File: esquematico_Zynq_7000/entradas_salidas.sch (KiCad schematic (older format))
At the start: 41 parts, among them U5 XC7Z010

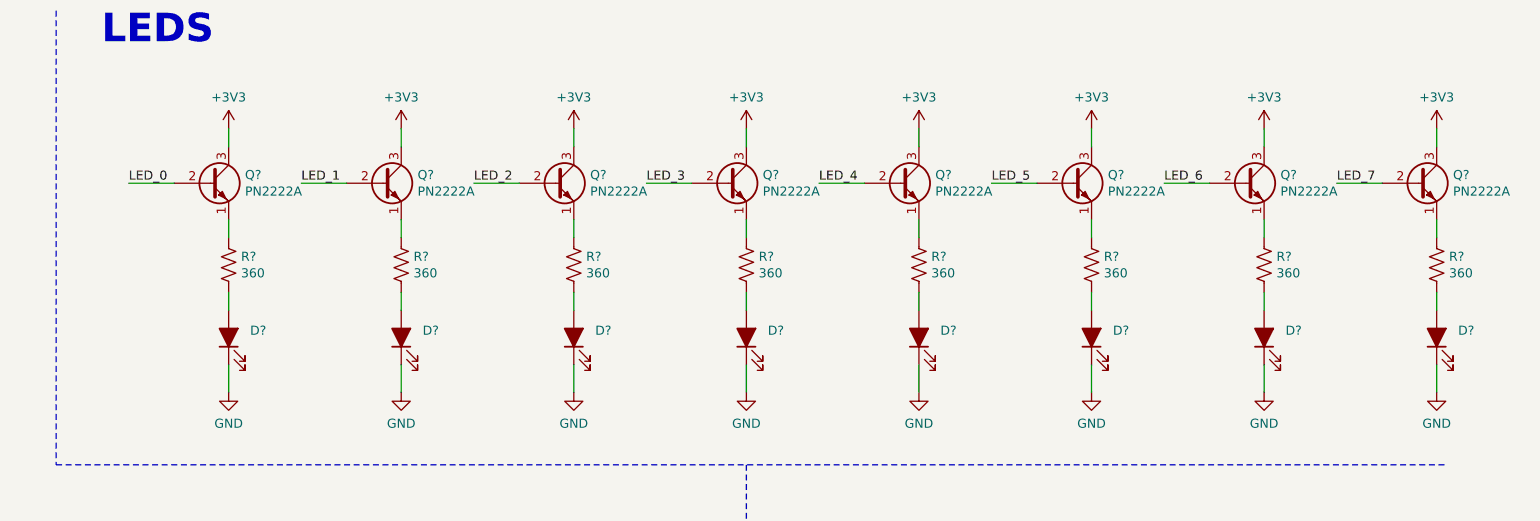
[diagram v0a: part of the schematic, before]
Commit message: upd
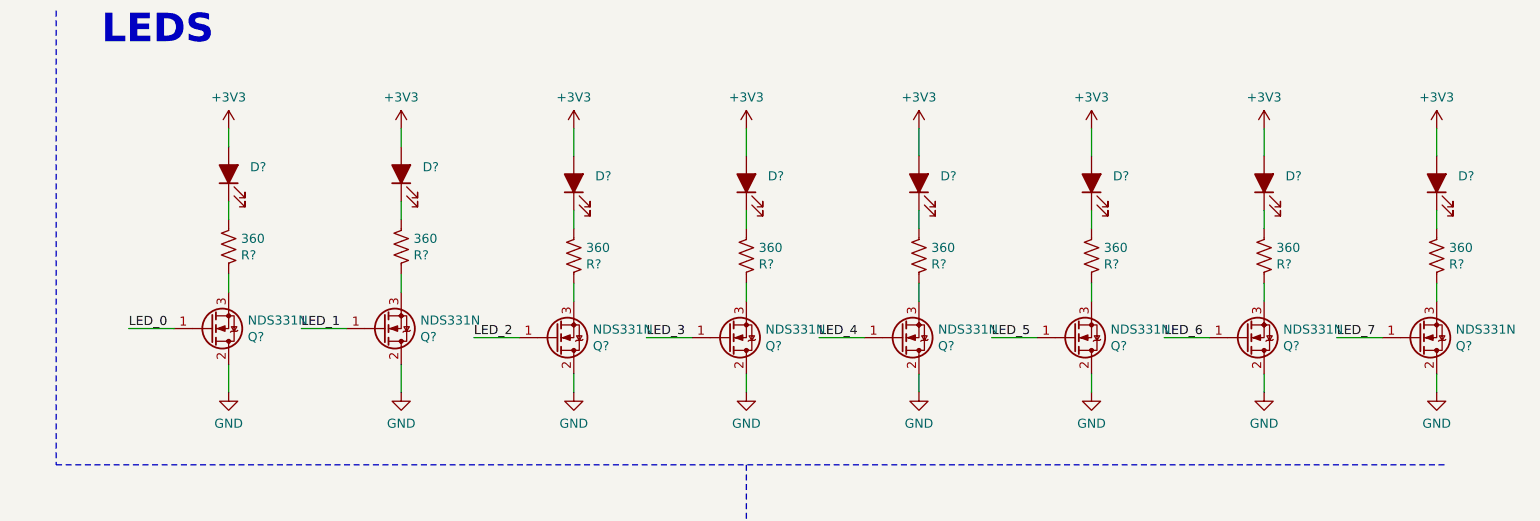
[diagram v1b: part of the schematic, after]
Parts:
- removed Q? (x8): PN2222A, Package_TO_SOT_THT:TO-92_Inline, symbol Transistor_BJT:PN2222A
- added Q? (x8): NDS331N, Package_TO_SOT_SMD:SOT-23, symbol Zynq_7000:NDS331N
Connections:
- net +3V3: now also D?.2 (A), D?.2 (A), D?.2 (A), D?.2 (A), D?.2 (A), D?.2 (A), D?.2 (A), D?.2 (A)
- net GND: now also Q?.2 (D), Q?.2 (D), Q?.2 (D), Q?.2 (D), Q?.2 (D), Q?.2 (D), Q?.2 (D), Q?.2 (D); no longer D?.1 (K), D?.1 (K), D?.1 (K), D?.1 (K), D?.1 (K), D?.1 (K), D?.1 (K), D?.1 (K)
- net LED_0: now also Q?.1 (G)
- net LED_1: now also Q?.1 (G)
- net LED_2: now also Q?.1 (G)
- net LED_3: now also Q?.1 (G)
- net LED_4: now also Q?.1 (G)
- net LED_5: now also Q?.1 (G)
- net LED_6: now also Q?.1 (G)
- net LED_7: now also Q?.1 (G)
- net at R?.2: now also D?.1 (K); no longer D?.2 (A) (x8)
- net at R?.1: now also Q?.3 (S) (x8)
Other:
- moved on the sheet: D?, R?
